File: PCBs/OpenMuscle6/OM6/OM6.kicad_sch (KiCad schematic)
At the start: 3 parts, among them U1 AH1806-P, U2 AH1806-P

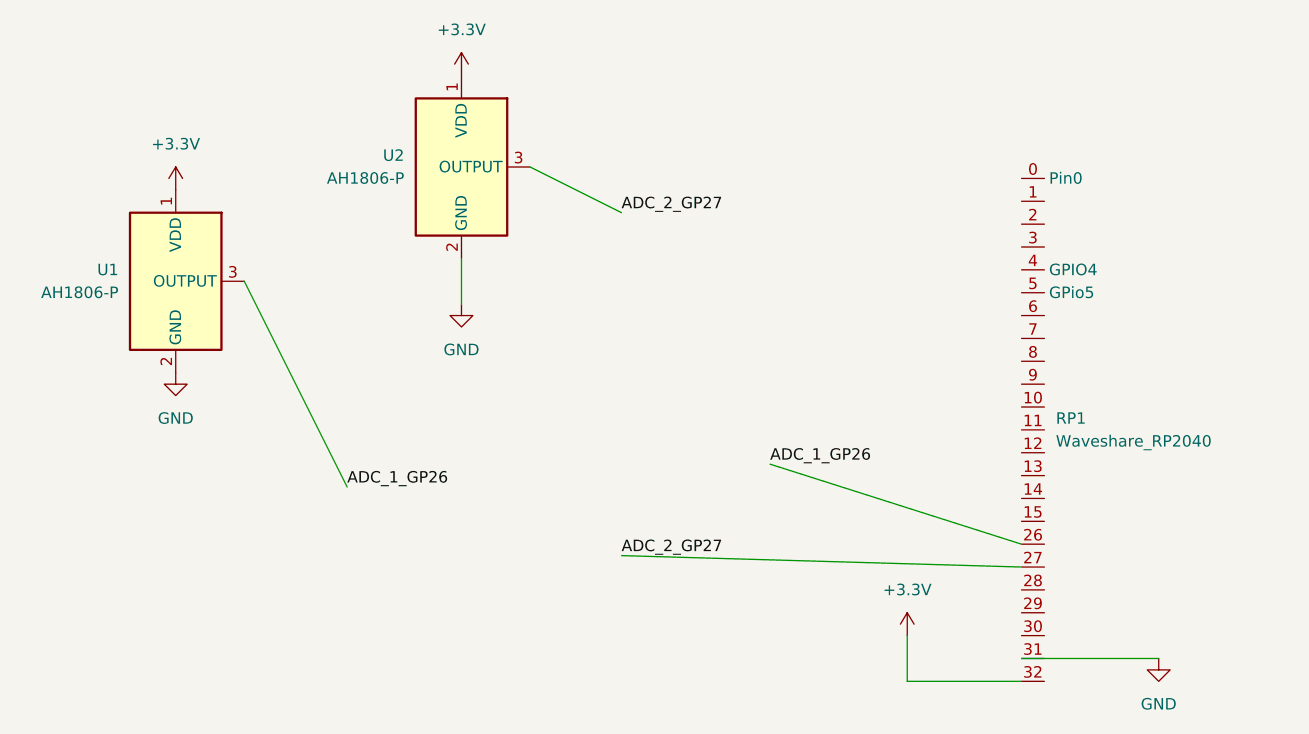
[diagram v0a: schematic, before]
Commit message: LASK4
Updates
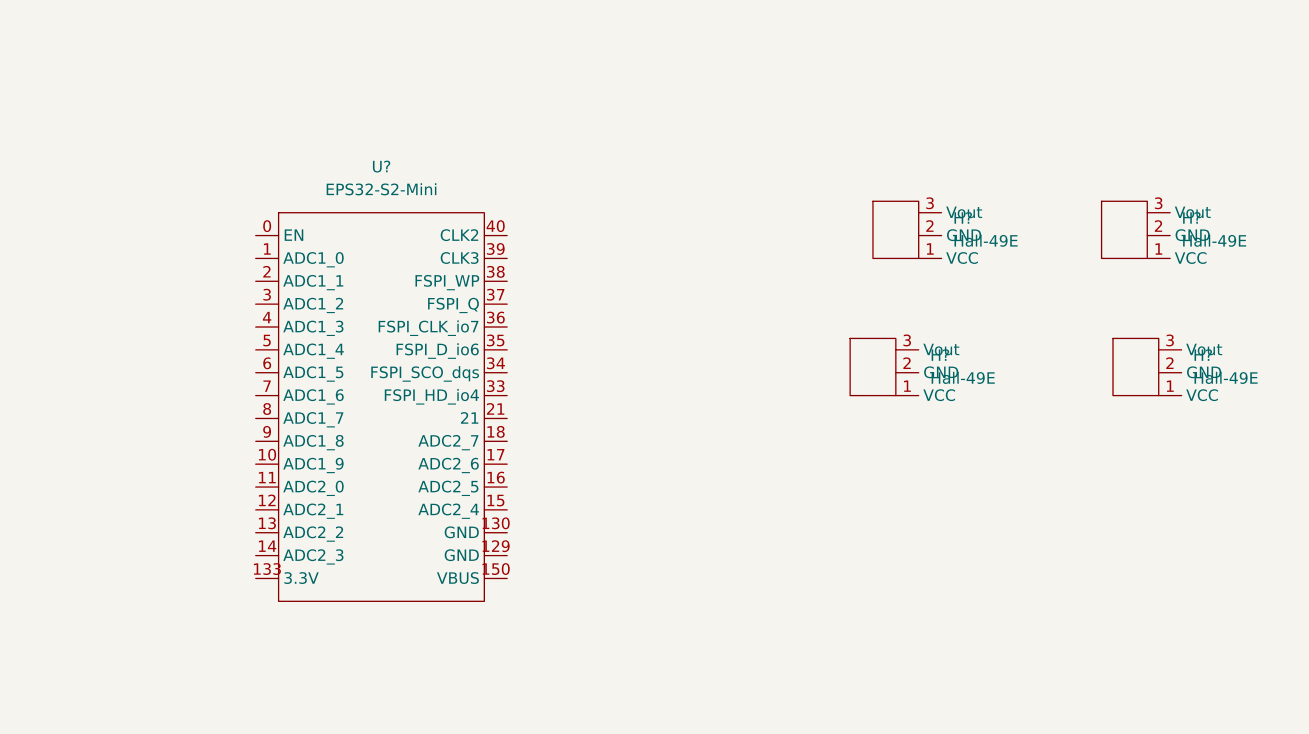
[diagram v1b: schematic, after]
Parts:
- removed RP1: Waveshare_RP2040, CustomTMFoot:RP2040-Zero, symbol TMOlib:Waveshare_RP2040
- removed U1, U2: AH1806-P, Connector_JST:JST_EH_B3B-EH-A_1x03_P2.50mm_Vertical, symbol Sensor_Magnetic:AH1806-P
- added H? (x4): Hall-49E, symbol OpenMuscleLibrary:Hall-49E
- added U?: EPS32-S2-Mini, symbol OpenMuscleLibrary:EPS32-S2-Mini
